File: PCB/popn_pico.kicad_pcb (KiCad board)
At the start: 2 copper layers, 180 x 100 mm, 39 parts, among them SW1 KAN4542-0701C, SW2 KAN4542-0701C, U1 Pico

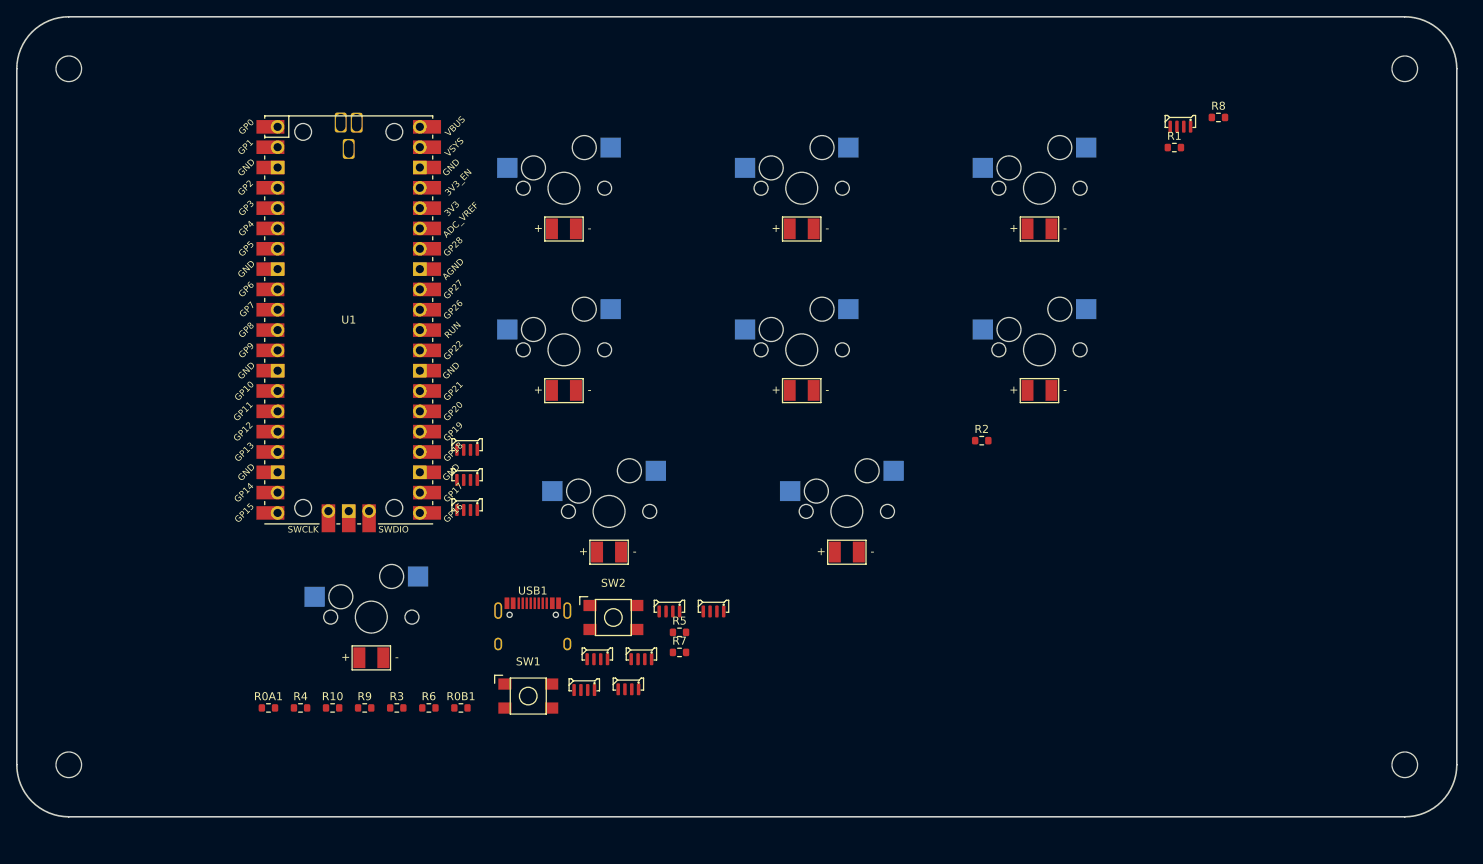
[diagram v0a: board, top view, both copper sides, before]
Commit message: Finished layout
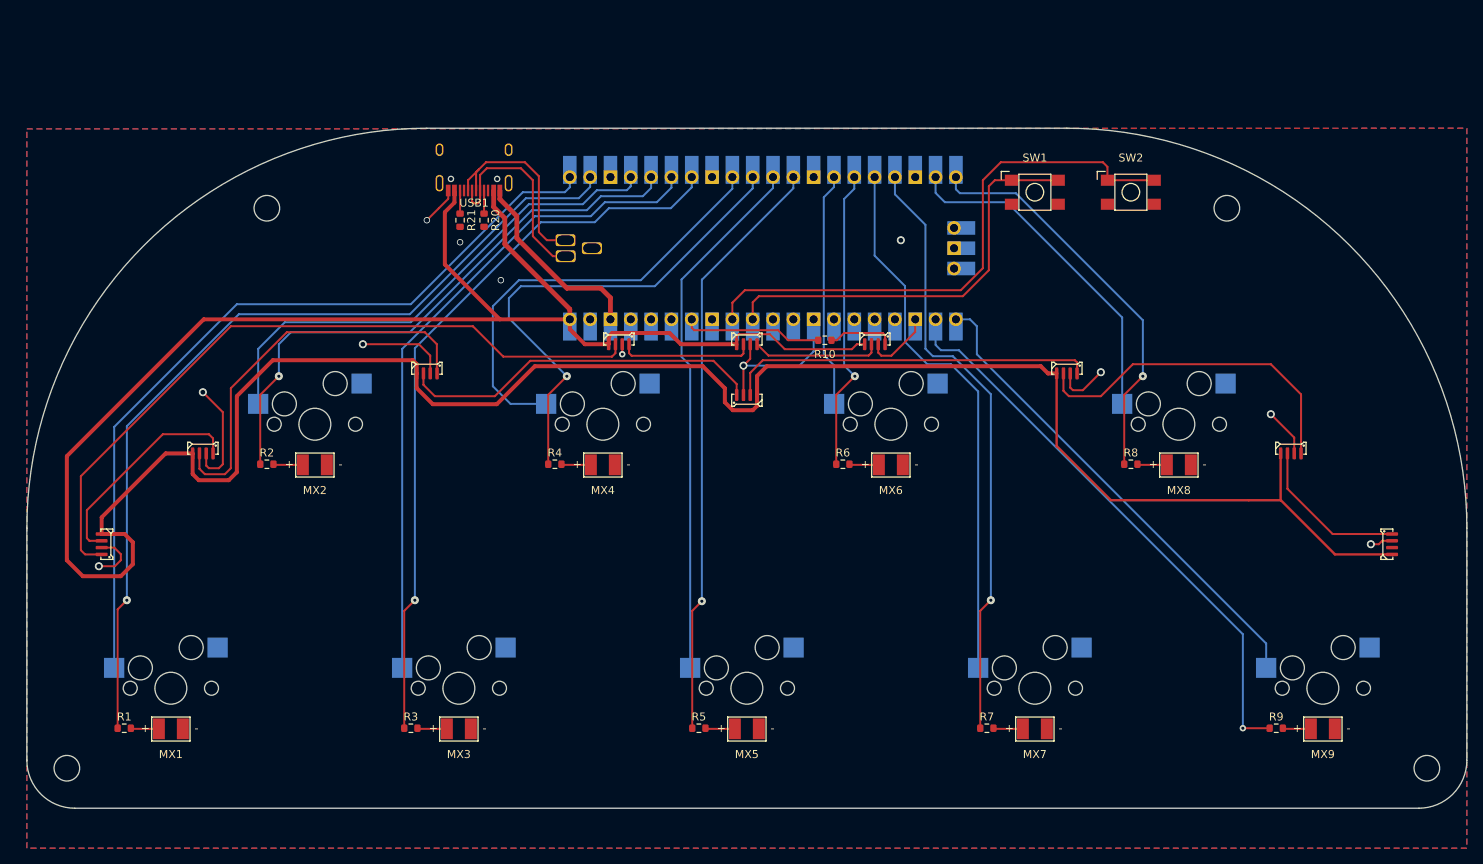
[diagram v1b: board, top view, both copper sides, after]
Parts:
- removed the REF** at (229.6, 55.0)
- removed the REF** at (62.6, 55.0)
- removed the REF** at (62.6, 142.0)
- added REF**: MountingHole_3.2mm_M3, MountingHole:MountingHole_3.2mm_M3, F.Cu at (232.3, 142.4)
- added REF**: MountingHole_3.2mm_M3, MountingHole:MountingHole_3.2mm_M3, F.Cu at (62.3, 142.4)
- added REF**: MountingHole_3.2mm_M3, MountingHole:MountingHole_3.2mm_M3, F.Cu at (207.3, 72.4)
- MX1: value MX-LED-B -> MX-BUTTON; footprint MX_Only:MXOnly-1.5U-Hotswap-LED-SMD -> MX_Only:MXOnly-Popn_Button-Hotswap-LED
- MX2, MX3, MX4, MX5: value MX-LED -> MX-BUTTON; footprint MX_Only:MXOnly-1.5U-Hotswap-LED-SMD -> MX_Only:MXOnly-Popn_Button-Hotswap-LED
- MX6, MX7, MX8, MX9: value MX-LED-R -> MX-BUTTON; footprint MX_Only:MXOnly-1.5U-Hotswap-LED-SMD -> MX_Only:MXOnly-Popn_Button-Hotswap-LED
- U1: footprint MCU_RaspberryPi_and_Boards:RPi_Pico_SMD_TH -> MCU_RaspberryPi_and_Boards:RPi_Pico_SMD; moved to B.Cu
- moved REF** 158.3 mm to (87.3, 72.4)
- moved R1 150.0 mm to (69.5, 137.4)
- moved LED4 144.2 mm to (67.3, 114.4), turned to -90 degrees
- moved R9 114.0 mm to (213.5, 137.4)
- moved LED9 103.0 mm to (215.3, 102.4)
- moved LED10 90.0 mm to (227.3, 114.4), turned to 90 degrees
- moved R2 89.4 mm to (87.3, 104.4)
- moved SW1 89.3 mm to (183.3, 70.4)
- moved SW2 83.7 mm to (195.3, 70.4)
- moved R10 76.8 mm to (157.1, 88.9)
- moved MX3 75.8 mm to (111.3, 132.4)
- moved LED8 75.6 mm to (187.3, 92.4)
- moved USB1 67.4 mm to (113.2, 62.5), turned to 180 degrees
- moved R20 66.7 mm to (114.5, 73.9), turned to -90 degrees
- moved MX7 62.5 mm to (183.3, 132.4)
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- renumbered R0A1 to R20, R0B1 to R21
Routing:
- net +5V: track 0.00 -> 398.0 mm
- net Net-(R1-Pad1): track 0.00 -> 109.8 mm, vias 0 -> 1
- net GND: track 0.00 -> 106.6 mm, vias 0 -> 12
- net Net-(MX1-Pad1): track 0.00 -> 100.8 mm
- net Net-(R3-Pad1): track 0.00 -> 92.3 mm, vias 0 -> 1
- net Net-(LED3-Pad3): track 0.00 -> 89.5 mm
- net Net-(MX3-Pad1): track 0.00 -> 83.2 mm
- net Net-(R7-Pad1): track 0.00 -> 75.9 mm, vias 0 -> 1
- net Net-(R5-Pad1): track 0.00 -> 74.1 mm, vias 0 -> 1
- net Net-(R2-Pad1): track 0.00 -> 71.9 mm, vias 0 -> 1
- net Net-(R9-Pad1): track 0.00 -> 71.7 mm, vias 0 -> 1
- net Net-(SW2-Pad1): track 0.00 -> 70.4 mm
- net Net-(MX7-Pad1): track 0.00 -> 68.4 mm
- net Net-(MX5-Pad1): track 0.00 -> 66.5 mm
- net Net-(MX2-Pad1): track 0.00 -> 63.0 mm
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- added copper zone on B.Cu, net GND
- added copper zone on F.Cu, net GND
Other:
- board size 180 x 100 mm -> 180 x 85 mm
